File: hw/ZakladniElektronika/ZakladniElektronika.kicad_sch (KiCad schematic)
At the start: 4 parts, among them J5 Conn_01x08, J6 Conn_01x08, J7 Conn_01x32, J8 Conn_01x32

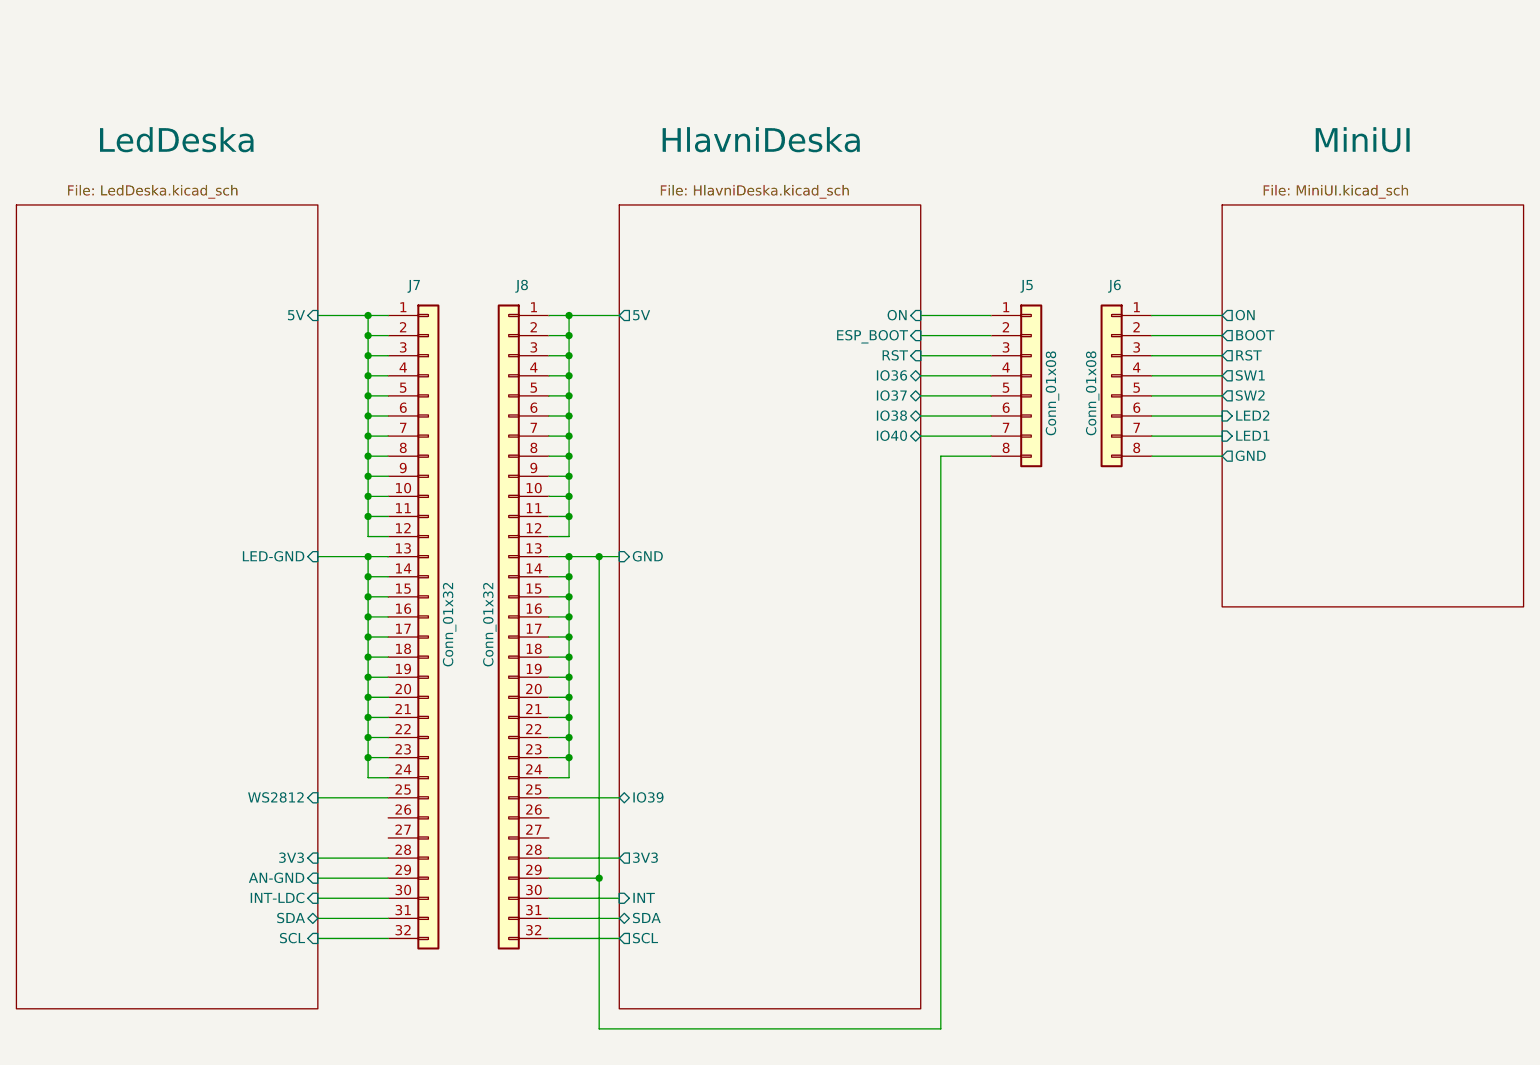
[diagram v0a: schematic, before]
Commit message: WIP
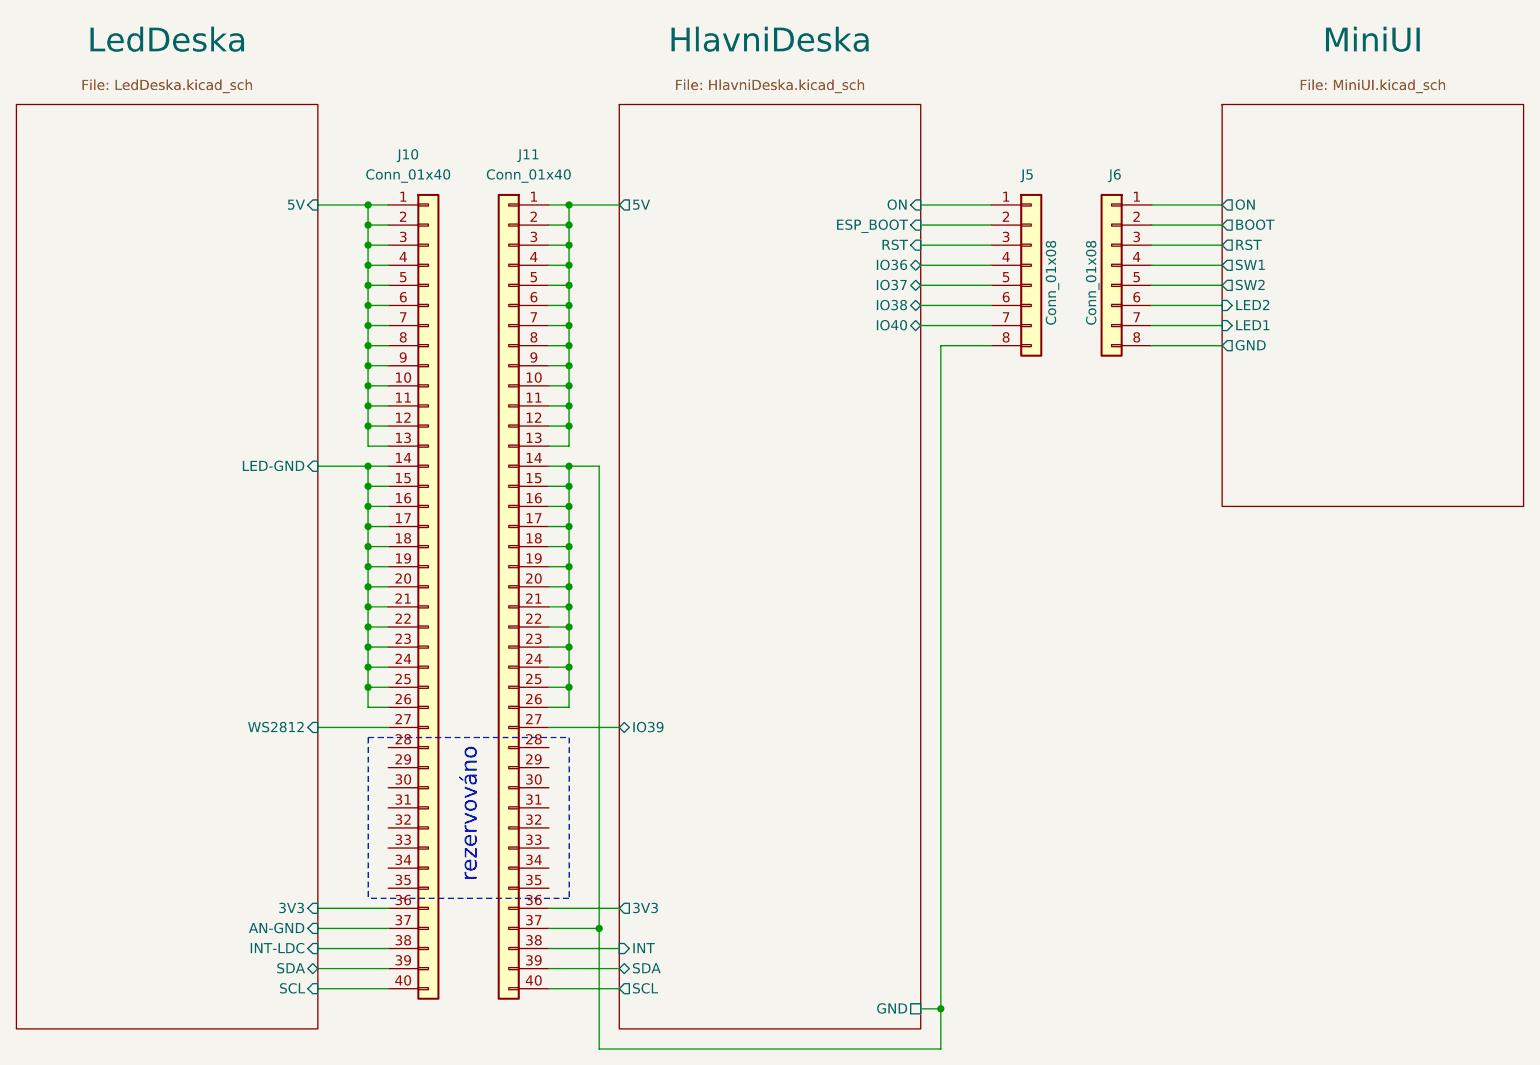
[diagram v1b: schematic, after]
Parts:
- removed J7, J8: Conn_01x32, Connector_FFC-FPC:TE_3-1734839-2_1x32-1MP_P0.5mm_Horizontal, symbol Connector_Generic:Conn_01x32
- added J10: Conn_01x40, Connector_FFC-FPC:Molex_52559-3652_2x18-1MP_P0.5mm_Vertical, symbol Connector_Generic:Conn_01x40
- added J11: Conn_01x40, Connector_FFC-FPC:Hirose_FH12-40S-0.5SH_1x40-1MP_P0.50mm_Horizontal, symbol Connector_Generic:Conn_01x40
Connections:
- net HlavniDeska/3V3: now also J11.36 (Pin_36)
- net HlavniDeska/5V: now also J11.1 (Pin_1), J11.10 (Pin_10), J11.11 (Pin_11), J11.12 (Pin_12), J11.13 (Pin_13), J11.2 (Pin_2), J11.3 (Pin_3), J11.4 (Pin_4), J11.5 (Pin_5), J11.6 (Pin_6), J11.7 (Pin_7), J11.8 (Pin_8), J11.9 (Pin_9)
- net HlavniDeska/GND: now also J11.14 (Pin_14), J11.15 (Pin_15), J11.16 (Pin_16), J11.17 (Pin_17), J11.18 (Pin_18), J11.19 (Pin_19), J11.20 (Pin_20), J11.21 (Pin_21), J11.22 (Pin_22), J11.23 (Pin_23), J11.24 (Pin_24), J11.25 (Pin_25), J11.26 (Pin_26), J11.37 (Pin_37)
- net HlavniDeska/INT: now also J11.38 (Pin_38)
- net HlavniDeska/IO39: now also J11.27 (Pin_27)
- net HlavniDeska/SCL: now also J11.40 (Pin_40)
- net HlavniDeska/SDA: now also J11.39 (Pin_39)
- net LedDeska/3V3: now also J10.36 (Pin_36)
- net LedDeska/5V: now also J10.1 (Pin_1), J10.10 (Pin_10), J10.11 (Pin_11), J10.12 (Pin_12), J10.13 (Pin_13), J10.2 (Pin_2), J10.3 (Pin_3), J10.4 (Pin_4), J10.5 (Pin_5), J10.6 (Pin_6), J10.7 (Pin_7), J10.8 (Pin_8), J10.9 (Pin_9)
- net LedDeska/AN-GND: now also J10.37 (Pin_37)
- net LedDeska/INT-LDC: now also J10.38 (Pin_38)
- net LedDeska/LED-GND: now also J10.14 (Pin_14), J10.15 (Pin_15), J10.16 (Pin_16), J10.17 (Pin_17), J10.18 (Pin_18), J10.19 (Pin_19), J10.20 (Pin_20), J10.21 (Pin_21), J10.22 (Pin_22), J10.23 (Pin_23), J10.24 (Pin_24), J10.25 (Pin_25), J10.26 (Pin_26)
- net LedDeska/SCL: now also J10.40 (Pin_40)
- net LedDeska/SDA: now also J10.39 (Pin_39)
- net LedDeska/WS2812: now also J10.27 (Pin_27)
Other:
- note added: "rezervováno"
- moved on the sheet: J5, J6
